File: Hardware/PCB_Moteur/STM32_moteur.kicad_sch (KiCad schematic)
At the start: 61 parts, among them J2 Conn_01x06_Pin, U2 STM32F103CBT6

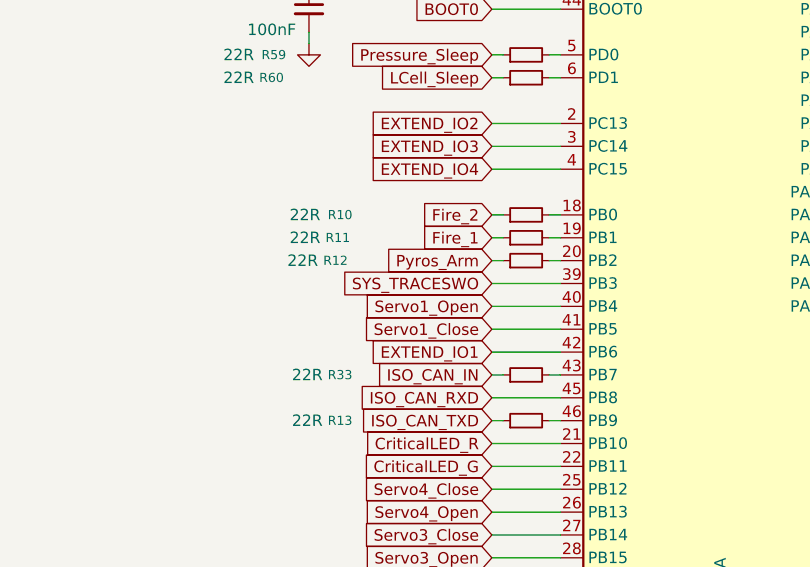
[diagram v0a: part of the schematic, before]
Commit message: wip: routing sys et limit switches
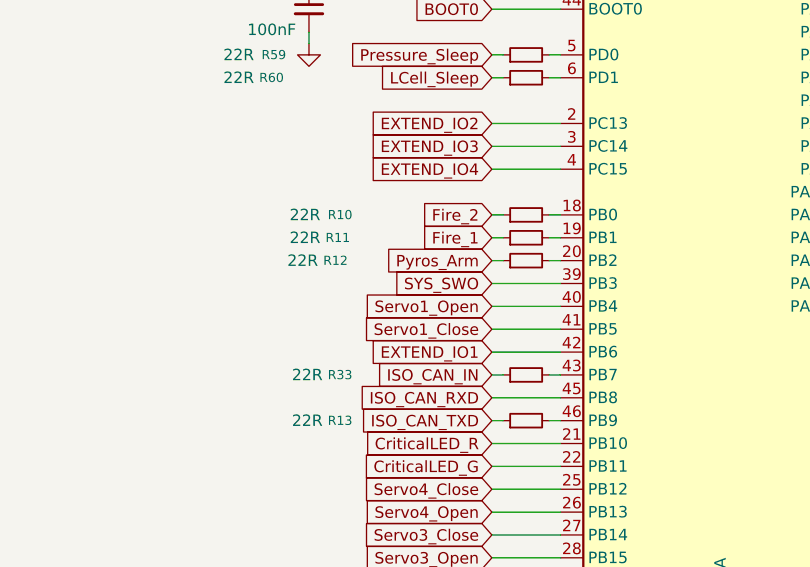
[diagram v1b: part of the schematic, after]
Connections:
- net SYS_TRACESWO is gone; now on net SYS_SWO: U2.39 (PB3)
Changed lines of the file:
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@@
 		)
 	)
-	(global_label "SYS_TRACESWO"
+	(global_label "SYS_SWO"
 		(shape input)
 		(at 125.73 87.63 180)
@@
 		)
 		(property "Intersheetrefs" "${INTERSHEET_REFS}"
-			(at 108.533 87.63 0)
+			(at 114.2782 87.63 0)
 			(effects
 				(font

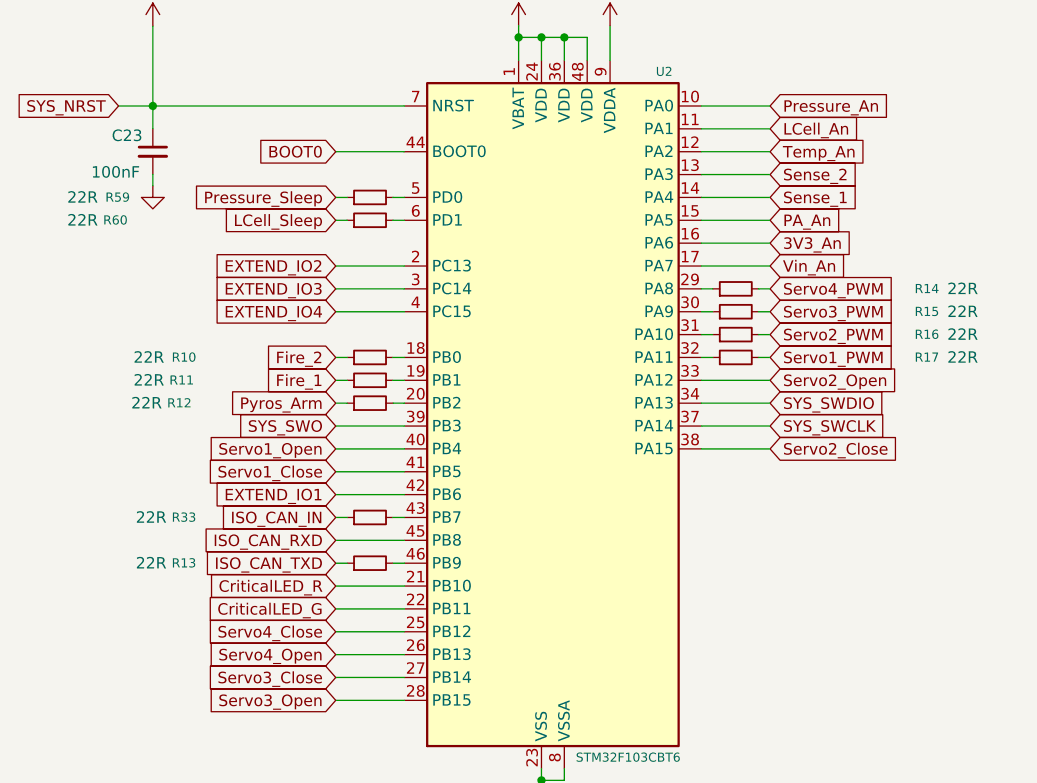
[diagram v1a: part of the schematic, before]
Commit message: wip: routing, bientot plane d'alim!
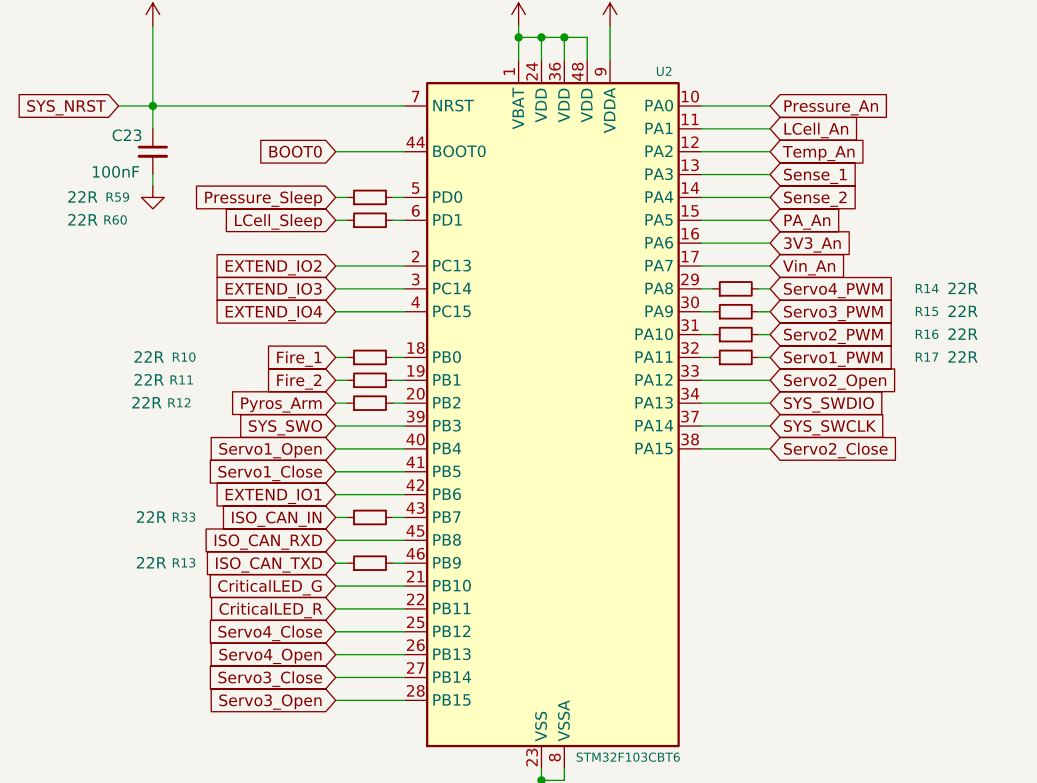
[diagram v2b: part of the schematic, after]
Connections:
- net CriticalLED_G: now also U2.21 (PB10); no longer U2.22 (PB11)
- net CriticalLED_R: now also U2.22 (PB11); no longer U2.21 (PB10)
- net Fire_1: now also R10.1; no longer R11.1
- net Fire_2: now also R11.1; no longer R10.1
- net Sense_1: now also U2.13 (PA3); no longer U2.14 (PA4)
- net Sense_2: now also U2.14 (PA4); no longer U2.13 (PA3)

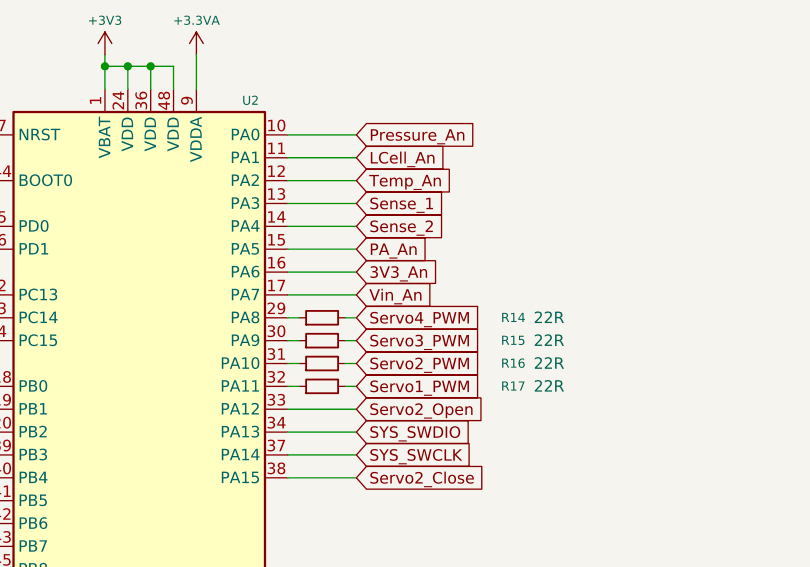
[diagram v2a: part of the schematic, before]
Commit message: wip: reste plane
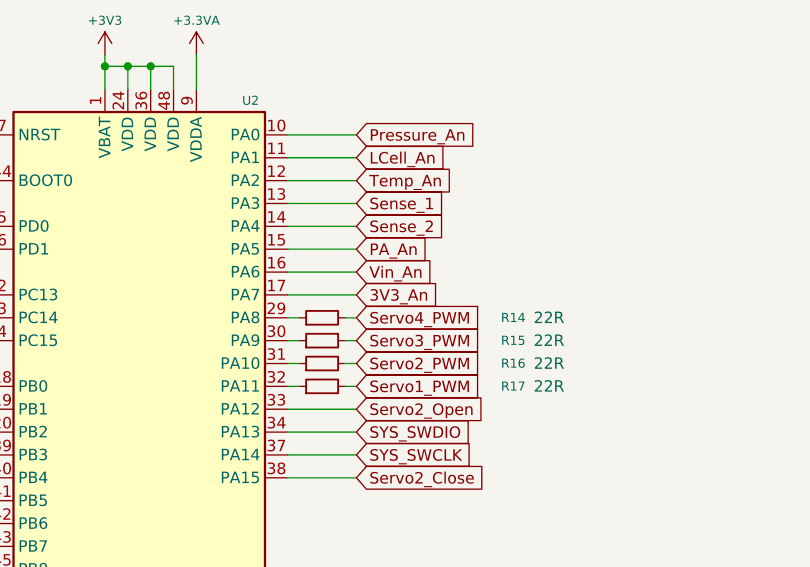
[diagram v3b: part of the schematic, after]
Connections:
- net 3V3_An: now also U2.17 (PA7); no longer U2.16 (PA6)
- net Vin_An: now also U2.16 (PA6); no longer U2.17 (PA7)
